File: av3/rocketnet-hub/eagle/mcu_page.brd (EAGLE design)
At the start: 112.7 x 76.2 mm, 274 parts, among them J1 ROCKETBUS, J2 ROCKETBUS, J3 ROCKETBUS, J4 ROCKETBUS, J5 ROCKETBUS, J6 ROCKETBUS, J7 ROCKETBUS, J8 ROCKETBUS, X1 87758-0416, X2 87758-0416, X3 87758-0416, X4 87758-0416, X5 87758-0416, X6 87758-0416, X7 87758-0416, X8 87758-0416

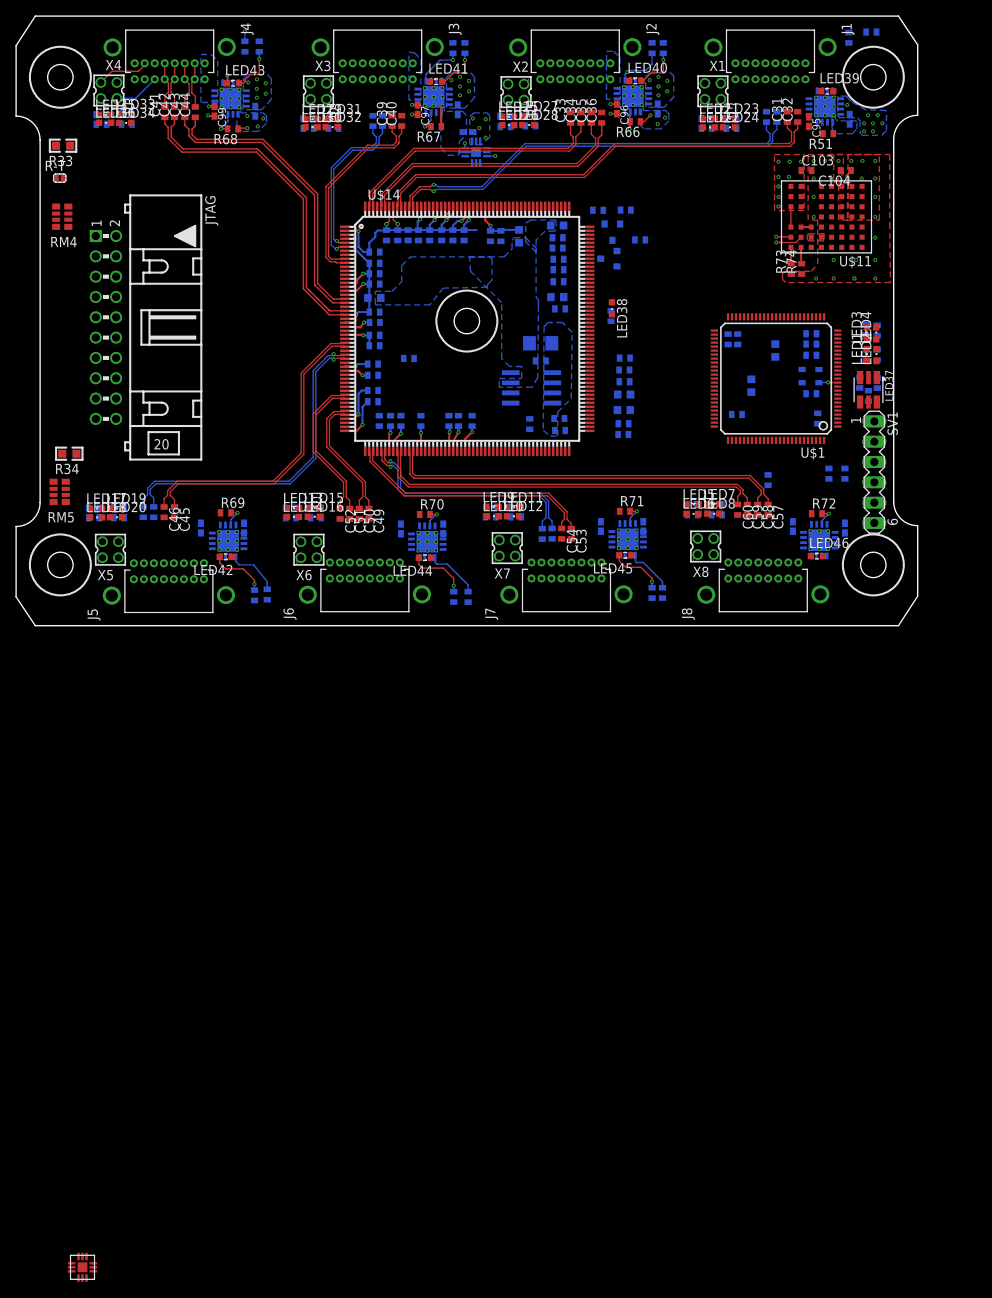
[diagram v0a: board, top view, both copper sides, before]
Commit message: more routing and layout work
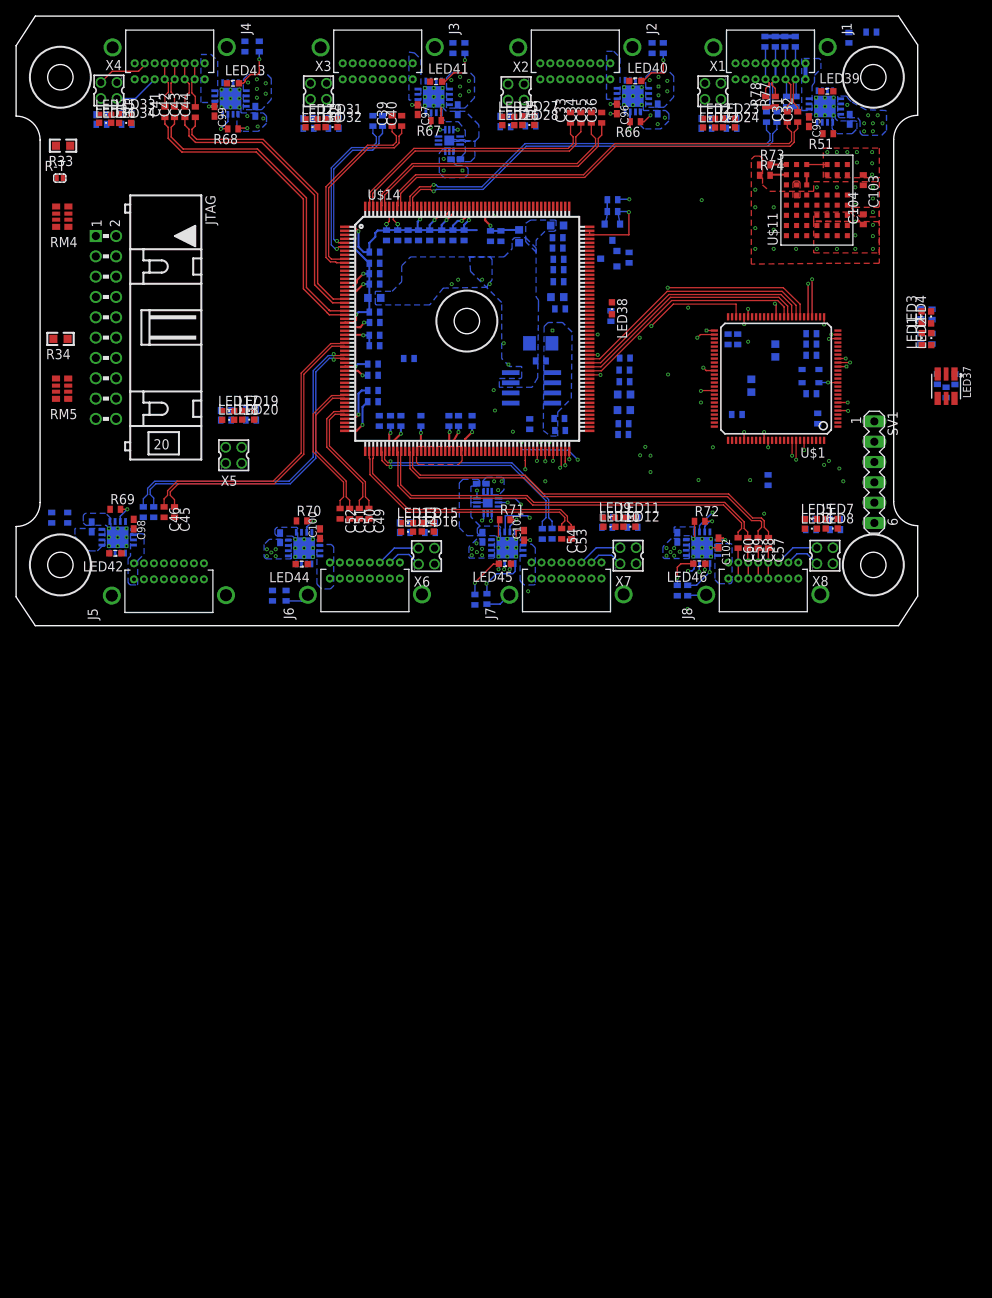
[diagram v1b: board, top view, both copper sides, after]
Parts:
- added C11: (no value), rcl:C0402K
- added R75, R76, R77, R78, R79, R80, R81, R82: (no value), rcl:R0402
- moved U$27 108.2 mm to (59.0, 15.4), flipped to the bottom, turned to 180 degrees
- moved R57 27.1 mm to (4.45, 13.5), turned to 90 degrees
- moved R56 26.7 mm to (6.45, 13.5), turned to 270 degrees
- moved R64 24.5 mm to (84.0, 4.40), turned to 90 degrees
- moved R65 23.9 mm to (82.7, 4.40), turned to 270 degrees
- moved R60 22.8 mm to (33.8, 3.75), turned to 90 degrees
- moved R61 22.7 mm to (32.0, 3.75)
- moved R63 22.2 mm to (57.4, 3.25)
- moved R62 22.0 mm to (58.9, 3.35)
- moved LED18 20.5 mm to (26.5, 25.7)
- moved LED19 20.5 mm to (29.0, 26.9)
- moved LED20 20.5 mm to (29.0, 25.8)
- moved R20 20.5 mm to (26.2, 26.9)
- moved R21 20.5 mm to (26.2, 25.7)
- moved R22 20.5 mm to (29.4, 27.0)
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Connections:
- removed net AUTOMDIX: U$1.37, U$14.87
- removed net CHASSIS: J1.CHASSIS@1, J1.CHASSIS@2, J2.CHASSIS@1, J2.CHASSIS@2, J3.CHASSIS@1, J3.CHASSIS@2, J4.CHASSIS@1, J4.CHASSIS@2, J5.CHASSIS@1, J5.CHASSIS@2, J6.CHASSIS@1, J6.CHASSIS@2, J7.CHASSIS@1, J7.CHASSIS@2, J8.CHASSIS@1, J8.CHASSIS@2
- removed net MODESEL0: U$1.91
- removed net MODESEL1: U$1.47, U$14.166
- removed net MODESEL2: U$1.53, U$14.165
- removed net MODESEL3: U$1.54, U$14.164, U$14.167
- removed net N$126: C91.2, U$7.5, U$7.DAP, U$7.P$10, U$7.P$2, U$7.P$3, U$7.P$4, U$7.P$5, U$7.P$6, U$7.P$7, U$7.P$8, U$7.P$9
- removed net N$127: C92.2, U$8.5, U$8.DAP, U$8.P$10, U$8.P$2, U$8.P$3, U$8.P$4, U$8.P$5, U$8.P$6, U$8.P$7, U$8.P$8, U$8.P$9
- removed net N$128: C93.2, U$9.5, U$9.DAP, U$9.P$10, U$9.P$2, U$9.P$3, U$9.P$4, U$9.P$5, U$9.P$6, U$9.P$7, U$9.P$8, U$9.P$9
- removed net N$129: C94.2, U$10.5, U$10.DAP, U$10.P$10, U$10.P$2, U$10.P$3, U$10.P$4, U$10.P$5, U$10.P$6, U$10.P$7, U$10.P$8, U$10.P$9
- removed net NODE1_IMON: U$1.25
- removed net NODE1_RXM: J1.USB_L@1
- removed net NODE1_RXP: J1.USB_H@1
- removed net NODE1_TXM: J1.CAN_L@1
- removed net NODE1_TXP: J1.CAN_H@1, J1.CAN_H@2
- removed net NODE2_IMON: U$1.29
- removed net NODE3_IMON: U$1.30
- removed net NODE4_IMON: U$1.31
- new net NODE1_TX_N: C31.2, J1.CAN_L@1, J1.CAN_L@2, R76.2, R80.1
- new net NODE5_8_IMON: U$1.16, U$27.P$8
- net +3V3: now also C11.1, R75.1, R76.1, R77.1, R78.1, U$27.P$4, U$27.P$6
- net GND: now also C11.2, C91.2, C92.2, C93.2, C94.2, J1.CHASSIS@1, J1.CHASSIS@2, J2.CHASSIS@1, J2.CHASSIS@2, J3.CHASSIS@1, J3.CHASSIS@2, J4.CHASSIS@1, J4.CHASSIS@2, J5.CHASSIS@1, J5.CHASSIS@2, J6.CHASSIS@1, J6.CHASSIS@2, J7.CHASSIS@1, J7.CHASSIS@2, J8.CHASSIS@1, J8.CHASSIS@2, R79.2, R80.2, R81.2, R82.2, U$10.5, U$10.DAP, U$10.P$10, U$10.P$2, U$10.P$3, U$10.P$4, U$10.P$5, U$10.P$6, U$10.P$7, U$10.P$8, U$10.P$9, U$27.P$13, U$27.P$2, U$7.5, U$7.DAP, U$7.P$10, U$7.P$2, U$7.P$3, U$7.P$4, U$7.P$5, U$7.P$6, U$7.P$7, U$7.P$8, U$7.P$9, U$8.5, U$8.DAP, U$8.P$10, U$8.P$2, U$8.P$3, U$8.P$4, U$8.P$5, U$8.P$6, U$8.P$7, U$8.P$8, U$8.P$9, U$9.5, U$9.DAP, U$9.P$10, U$9.P$2, U$9.P$3, U$9.P$4, U$9.P$5, U$9.P$6, U$9.P$7, U$9.P$8, U$9.P$9
- net IMON_A0: now also U$1.29, U$27.P$12
- net IMON_A1: now also U$1.30, U$27.P$10
- net MIIS0: no longer U$14.163
- net MIIS1: no longer U$14.162
- net MTXD0: no longer U$14.99
- net MTXD1: now also U$14.99; no longer U$14.98
- net MTXD2: now also U$14.98
- net NODE1_4_IMON: now also U$1.15
- net NODE1_RX_N: now also J1.USB_L@1, J1.USB_L@2, R78.2, R82.1
- net NODE1_RX_P: now also J1.USB_H@1, J1.USB_H@2, R77.2, R81.1
- net NODE1_TX_P: now also J1.CAN_H@1, J1.CAN_H@2, R75.2, R79.1; no longer C31.2
- net NODE5_IMON: now also U$27.P$1; no longer U$1.15
- net NODE6_IMON: now also U$27.P$9; no longer U$1.16
- net NODE7_IMON: now also U$27.P$3
- net NODE8_IMON: now also U$27.P$7
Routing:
- net IMON_A1: track 0.00 -> 100.5 mm, vias 0 -> 5
- net IMON_A0: track 0.00 -> 99.5 mm, vias 0 -> 5
- net NODE7_!EN: track 0.00 -> 66.4 mm, vias 0 -> 3
- net NODE7_!FLT: track 0.00 -> 64.9 mm, vias 0 -> 4
- net NODE5_8_IMON: track 0.00 -> 61.9 mm, vias 0 -> 3
- net MTXD2: track 0.00 -> 60.0 mm, vias 0 -> 4
- net MCOL: track 0.00 -> 52.7 mm, vias 0 -> 3
- net MTXC: track 0.00 -> 52.4 mm, vias 0 -> 3
- net MCRS: track 0.00 -> 50.7 mm, vias 0 -> 3
- net 25MHZ_REF_CLK: track 0.00 -> 50.6 mm, vias 0 -> 3
- net NODE7_!PG: track 0.00 -> 48.9 mm, vias 0 -> 3
- net NODE8_!EN: track 0.00 -> 47.2 mm, vias 0 -> 3
- net NODE8_IMON: track 0.00 -> 46.3 mm, vias 0 -> 4
- net NODE7_LTCH: track 0.00 -> 46.2 mm, vias 0 -> 3
- net MTXEN: track 0.00 -> 45.3 mm, vias 0 -> 3
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- added copper zone on layer 15, net +3V3
- added copper zone on layer 16, net NODE1_VOUT
- added copper zone on layer 16, net NODE5_VOUT
- added copper zone on layer 16, net NODE6_VOUT
- added copper zone on layer 16, net NODE7_VOUT
- added copper zone on layer 16, net NODE8_VOUT
- removed copper zone on layer 15, net TEMP
